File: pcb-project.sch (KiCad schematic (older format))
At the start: 146 parts, among them SW1 SW_PUSH, U2 ATMEGA32U4, X2 XTAL_GND

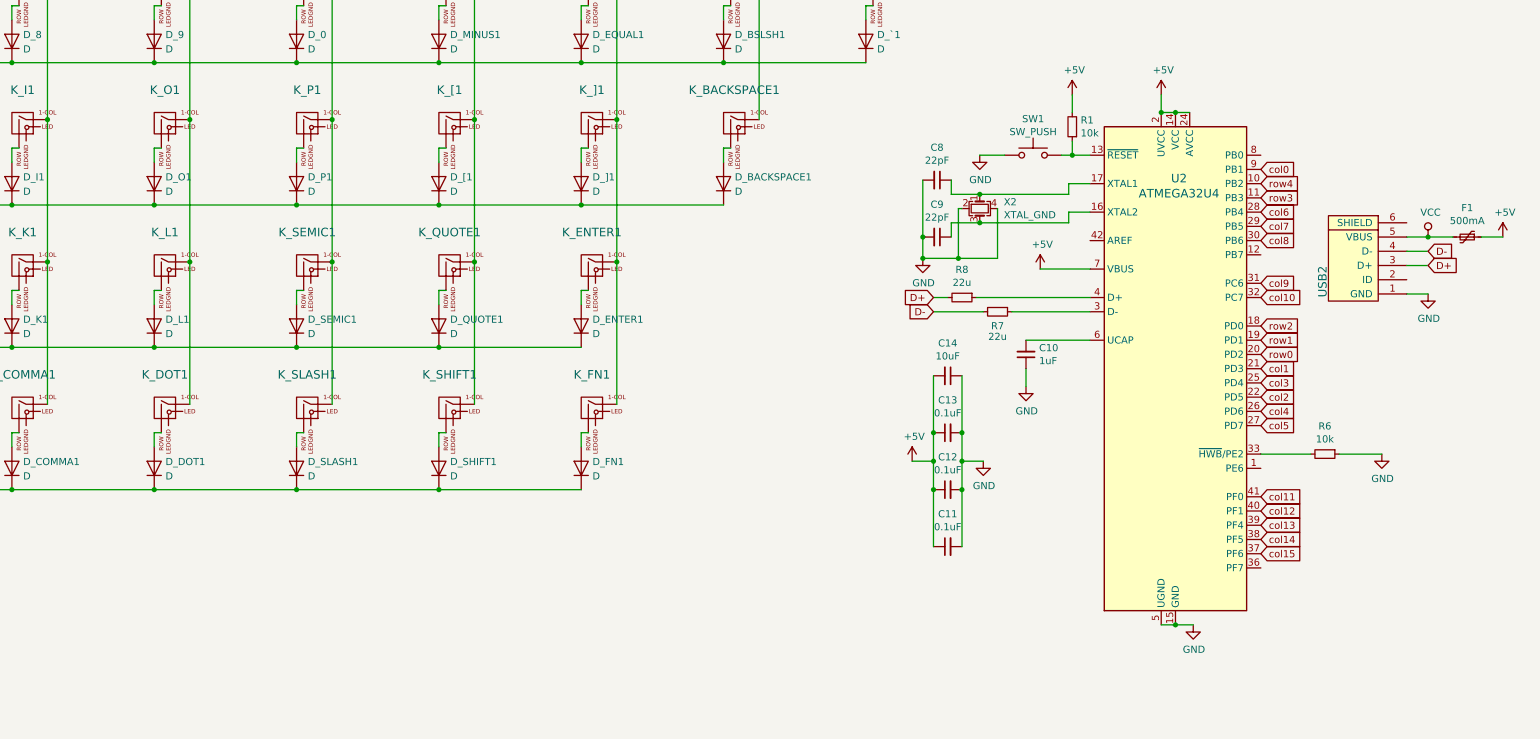
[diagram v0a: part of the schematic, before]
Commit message: Schematic Update For RGB
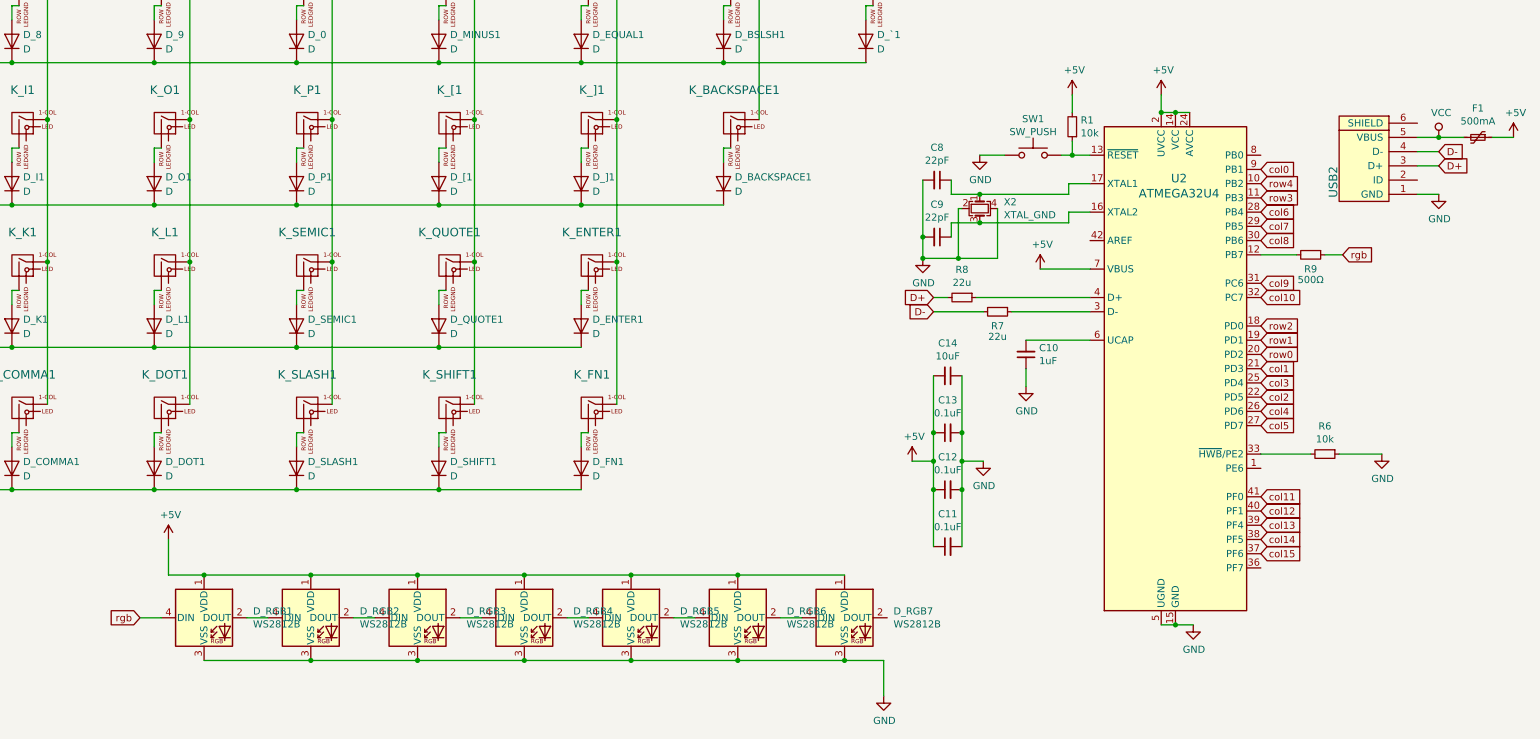
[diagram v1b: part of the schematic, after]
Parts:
- added D_RGB1, D_RGB2, D_RGB3, D_RGB4, D_RGB5, D_RGB6, D_RGB7: WS2812B, LED_SMD:LED_WS2812B_PLCC4_5.0x5.0mm_P3.2mm, symbol LED:WS2812B
- added R9: 500Ω, Resistor_SMD:R_0805_2012Metric, symbol Device:R_Small
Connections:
- net +5V: now also D_RGB1.1 (VDD), D_RGB2.1 (VDD), D_RGB3.1 (VDD), D_RGB4.1 (VDD), D_RGB5.1 (VDD), D_RGB6.1 (VDD), D_RGB7.1 (VDD)
- net GND: now also D_RGB1.3 (VSS), D_RGB2.3 (VSS), D_RGB3.3 (VSS), D_RGB4.3 (VSS), D_RGB5.3 (VSS), D_RGB6.3 (VSS), D_RGB7.3 (VSS)
- net at U2.12 (PB7): now also R9.2
- new net: D_RGB6.2 (DOUT), D_RGB7.4 (DIN)
- new net: D_RGB5.2 (DOUT), D_RGB6.4 (DIN)
- new net: D_RGB4.2 (DOUT), D_RGB5.4 (DIN)
- new net: D_RGB3.2 (DOUT), D_RGB4.4 (DIN)
- new net: D_RGB2.2 (DOUT), D_RGB3.4 (DIN)
- new net: D_RGB1.2 (DOUT), D_RGB2.4 (DIN)
- new net rgb: D_RGB1.4 (DIN), R9.1
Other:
- moved on the sheet: F1, USB2
